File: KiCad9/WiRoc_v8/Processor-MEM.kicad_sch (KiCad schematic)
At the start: 28 parts

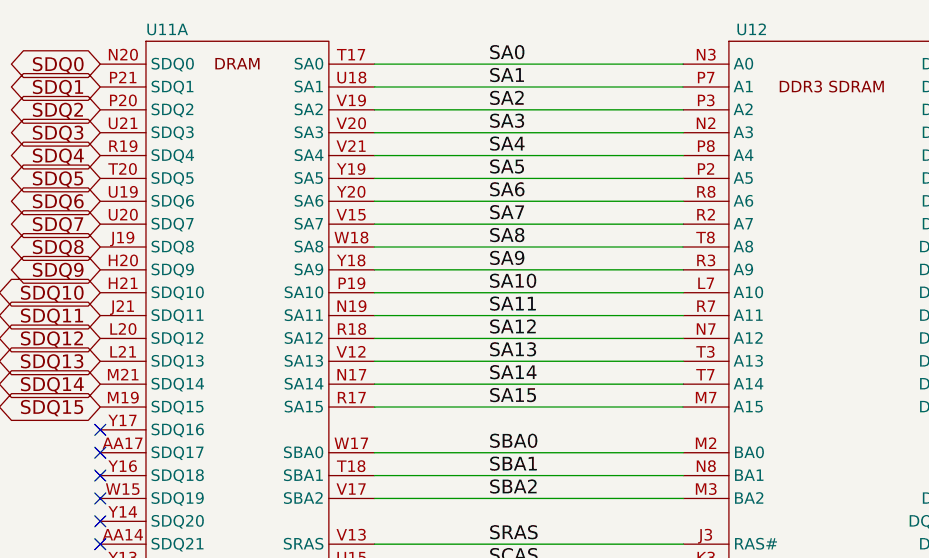
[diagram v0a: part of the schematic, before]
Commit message: etc
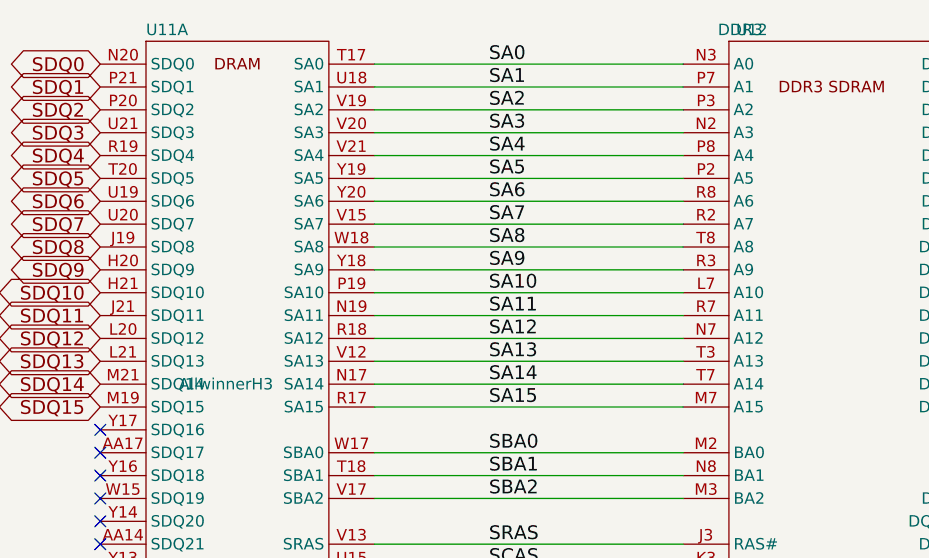
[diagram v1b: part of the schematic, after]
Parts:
- C46, C52: LCSC Part # (none) -> C15525; Manufacturer (none) -> Samsung Electro-Mechanics; ManufacturerPartNumber (none) -> CL05A106MQ5NUNC
- C47, C48, C53, C54, C58, C59: LCSC Part # (none) -> C52923; Manufacturer (none) -> Samsung Electro-Mechanics; ManufacturerPartNumber (none) -> CL05A105KA5NQNC
- U11: value ~ -> AllwinnerH3
- U12: value ~ -> DDR3
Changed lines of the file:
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@@
 			)
 		)
-		(property "Datasheet" "~"
+		(property "Datasheet" "https://jlcpcb.com/api/file/downloadByFileSystemAccessId/8579707174974914560"
 			(at 218.44 43.18 0)
 			(effects
@@
 		)
 		(property "Description" ""
+			(at 218.44 43.18 0)
+			(effects
+				(font
+					(size 1.27 1.27)
+				)
+				(hide yes)
+			)
+		)
+		(property "LCSC Part #" "C52923"
+			(at 218.44 43.18 0)
+			(effects
+				(font
+					(size 1.27 1.27)
+				)
+				(hide yes)
+			)
+		)
+		(property "Manufacturer" "Samsung Electro-Mechanics"
+			(at 218.44 43.18 0)
+			(effects
+				(font
+					(size 1.27 1.27)
+				)
+				(hide yes)
+			)
+		)
+		(property "ManufacturerPartNumber" "CL05A105KA5NQNC"
 			(at 218.44 43.18 0)
 			(effects
@@
 			)
 		)
-		(property "Datasheet" "~"
+		(property "Datasheet" "https://jlcpcb.com/api/file/downloadByFileSystemAccessId/8579707174974914560"
 			(at 207.01 91.44 0)
 			(effects
@@
 		)
 		(property "Description" ""
+			(at 207.01 91.44 0)
+			(effects
+				(font
+					(size 1.27 1.27)
+				)
+				(hide yes)
+			)
+		)
+		(property "LCSC Part #" "C52923"
+			(at 207.01 91.44 0)
+			(effects
+				(font
+					(size 1.27 1.27)
+				)
+				(hide yes)
+			)
+		)
+		(property "Manufacturer" "Samsung Electro-Mechanics"
+			(at 207.01 91.44 0)
+			(effects
+				(font
+					(size 1.27 1.27)
+				)
+				(hide yes)
+			)
+		)
+		(property "ManufacturerPartNumber" "CL05A105KA5NQNC"
 			(at 207.01 91.44 0)
 			(effects
@@
 			)
 		)
-		(property "Datasheet" "~"
+		(property "Datasheet" "https://jlcpcb.com/api/file/downloadByFileSystemAccessId/8579707174974914560"
 			(at 229.87 43.18 0)
 			(effects
@@
 		)
 		(property "Description" ""
+			(at 229.87 43.18 0)
+			(effects
+				(font
+					(size 1.27 1.27)
+				)
+				(hide yes)
+			)
+		)
+		(property "LCSC Part #" "C52923"
+			(at 229.87 43.18 0)
+			(effects
+				(font
+					(size 1.27 1.27)
+				)
+				(hide yes)
+			)
+		)
+		(property "Manufacturer" "Samsung Electro-Mechanics"
+			(at 229.87 43.18 0)
+			(effects
+				(font
+					(size 1.27 1.27)
+				)
+				(hide yes)
+			)
+		)
+		(property "ManufacturerPartNumber" "CL05A105KA5NQNC"
 			(at 229.87 43.18 0)
 			(effects
@@
 			)
 		)
+		(property "LCSC Part #" "C15525"
+			(at 207.01 67.31 0)
+			(effects
+				(font
+					(size 1.27 1.27)
+				)
+				(hide yes)
+			)
+		)
+		(property "Manufacturer" "Samsung Electro-Mechanics"
+			(at 207.01 67.31 0)
+			(effects
+				(font
+					(size 1.27 1.27)
+				)
+				(hide yes)
+			)
+		)
+		(property "ManufacturerPartNumber" "CL05A106MQ5NUNC"
+			(at 207.01 67.31 0)
+			(effects
+				(font
+					(size 1.27 1.27)
+				)
+				(hide yes)
+			)
+		)
 		(pin "2"
 		)
@@
 			)
 		)
-		(property "Datasheet" "~"
+		(property "Datasheet" "https://jlcpcb.com/api/file/downloadByFileSystemAccessId/8579707174974914560"
 			(at 229.87 67.31 0)
 			(effects
@@
 		)
 		(property "Description" ""
+			(at 229.87 67.31 0)
+			(effects
+				(font
+					(size 1.27 1.27)
+				)
+				(hide yes)
+			)
+		)
+		(property "LCSC Part #" "C52923"
+			(at 229.87 67.31 0)
+			(effects
+				(font
+					(size 1.27 1.27)
+				)
+				(hide yes)
+			)
+		)
+		(property "Manufacturer" "Samsung Electro-Mechanics"
+			(at 229.87 67.31 0)
+			(effects
+				(font
+					(size 1.27 1.27)
+				)
+				(hide yes)
+			)
+		)
+		(property "ManufacturerPartNumber" "CL05A105KA5NQNC"
 			(at 229.87 67.31 0)
 			(effects
@@
 			)
 		)
+		(property "LCSC Part #" "C15525"
+			(at 207.01 43.18 0)
+			(effects
+				(font
+					(size 1.27 1.27)
+				)
+				(hide yes)
+			)
+		)
+		(property "Manufacturer" "Samsung Electro-Mechanics"
+			(at 207.01 43.18 0)
+			(effects
+				(font
+					(size 1.27 1.27)
+				)
+				(hide yes)
+			)
+		)
+		(property "ManufacturerPartNumber" "CL05A106MQ5NUNC"
+			(at 207.01 43.18 0)
+			(effects
+				(font
+					(size 1.27 1.27)
+				)
+				(hide yes)
+			)
+		)
 		(pin "2"
 		)
@@
 			)
 		)
-		(property "Datasheet" "~"
+		(property "Datasheet" "https://jlcpcb.com/api/file/downloadByFileSystemAccessId/8579707174974914560"
 			(at 218.44 91.44 0)
 			(effects
@@
 		)
 		(property "Description" ""
+			(at 218.44 91.44 0)
+			(effects
+				(font
+					(size 1.27 1.27)
+				)
+				(hide yes)
+			)
+		)
+		(property "LCSC Part #" "C52923"
+			(at 218.44 91.44 0)
+			(effects
+				(font
+					(size 1.27 1.27)
+				)
+				(hide yes)
+			)
+		)
+		(property "Manufacturer" "Samsung Electro-Mechanics"
+			(at 218.44 91.44 0)
+			(effects
+				(font
+					(size 1.27 1.27)
+				)
+				(hide yes)
+			)
+		)
+		(property "ManufacturerPartNumber" "CL05A105KA5NQNC"
 			(at 218.44 91.44 0)
 			(effects
@@
 			)
 		)
-		(property "Datasheet" "~"
+		(property "Datasheet" "https://jlcpcb.com/api/file/downloadByFileSystemAccessId/8579707174974914560"
 			(at 218.44 67.31 0)
 			(effects
@@
 		)
 		(property "Description" ""
+			(at 218.44 67.31 0)
+			(effects
+				(font
+					(size 1.27 1.27)
+				)
+				(hide yes)
+			)
+		)
+		(property "LCSC Part #" "C52923"
+			(at 218.44 67.31 0)
+			(effects
+				(font
+					(size 1.27 1.27)
+				)
+				(hide yes)
+			)
+		)
+		(property "Manufacturer" "Samsung Electro-Mechanics"
+			(at 218.44 67.31 0)
+			(effects
+				(font
+					(size 1.27 1.27)
+				)
+				(hide yes)
+			)
+		)
+		(property "ManufacturerPartNumber" "CL05A105KA5NQNC"
 			(at 218.44 67.31 0)
 			(effects
@@
 			)
 		)
-		(property "Value" "~"
+		(property "Value" "DDR3"
 			(at 102.87 25.4 0)
 			(effects
@@
 			)
 		)
-		(property "Value" "~"
+		(property "Value" "AllwinnerH3"
 			(at 45.72 64.77 0)
 			(effects
